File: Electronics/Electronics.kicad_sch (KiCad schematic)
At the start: 54 parts, among them J1 MOT_L, J2 MOT_R, P1 USB_C_Plug_USB2.0, SW1 RST, SW10 BTN8, SW11 BTN9, SW2 BOOT, SW3 BTN1, SW4 BTN2, SW5 BTN3, SW6 BTN4, SW7 BTN5, SW8 BTN6, SW9 BTN7, U1 ESP32-S3-WROOM-1, U2 BMI270, U5 BMI270, U6 NCP1117-3.3_SOT223, U7 NCP1117-3.3_SOT223

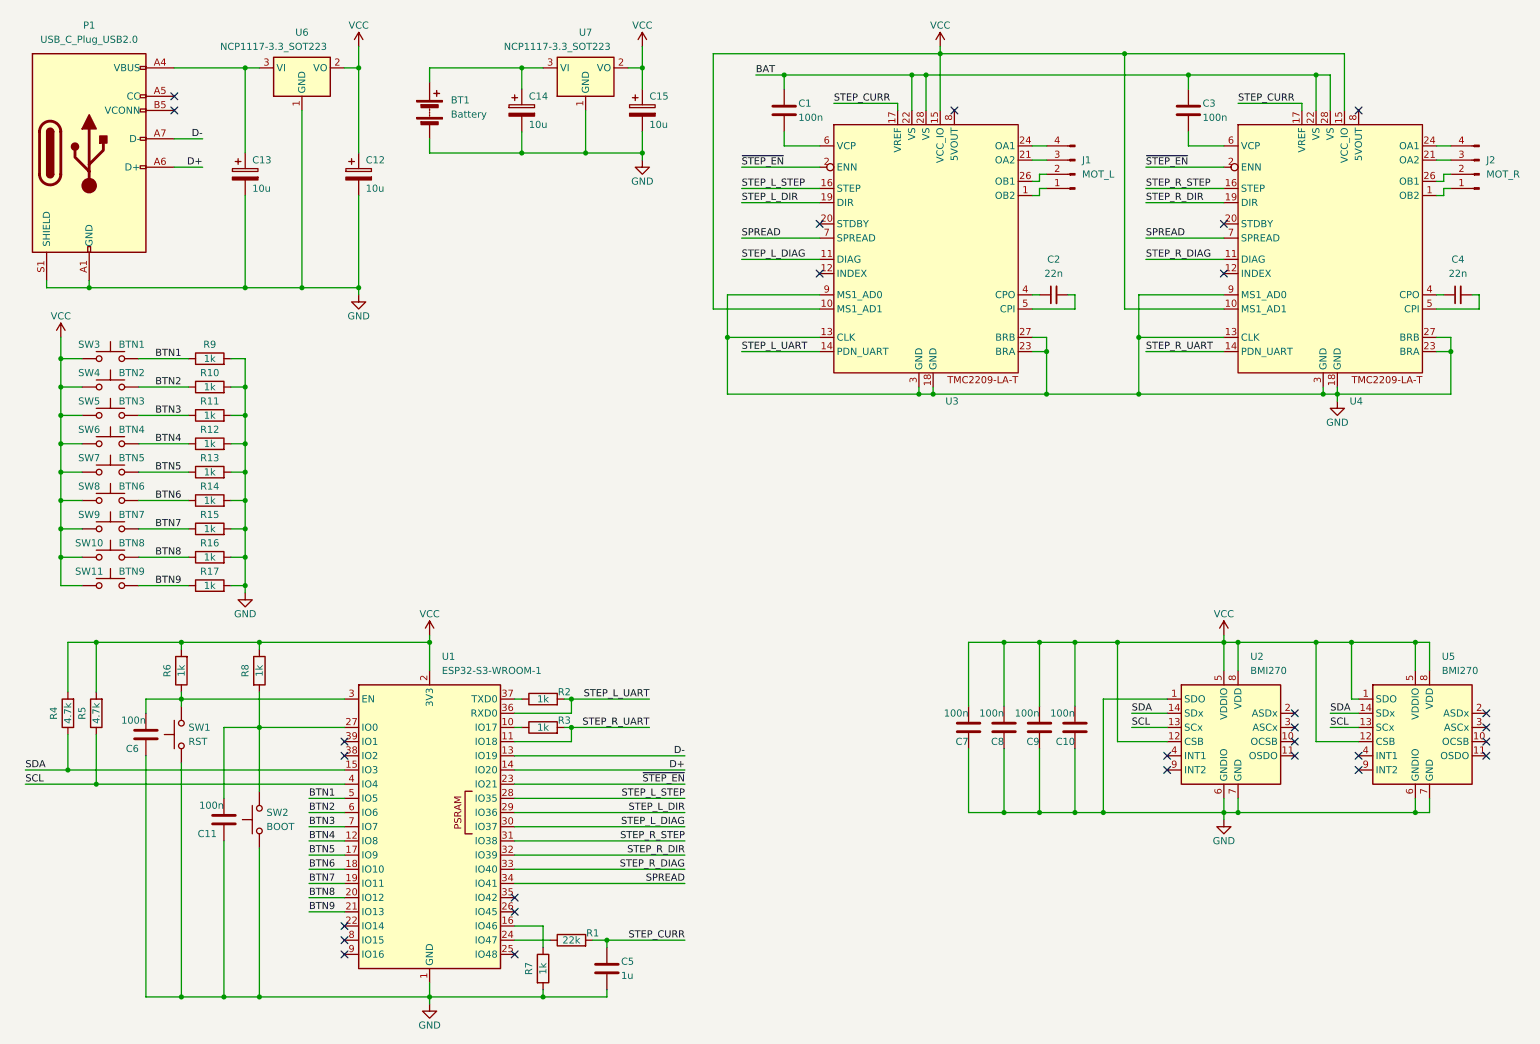
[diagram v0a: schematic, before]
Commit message: oleds
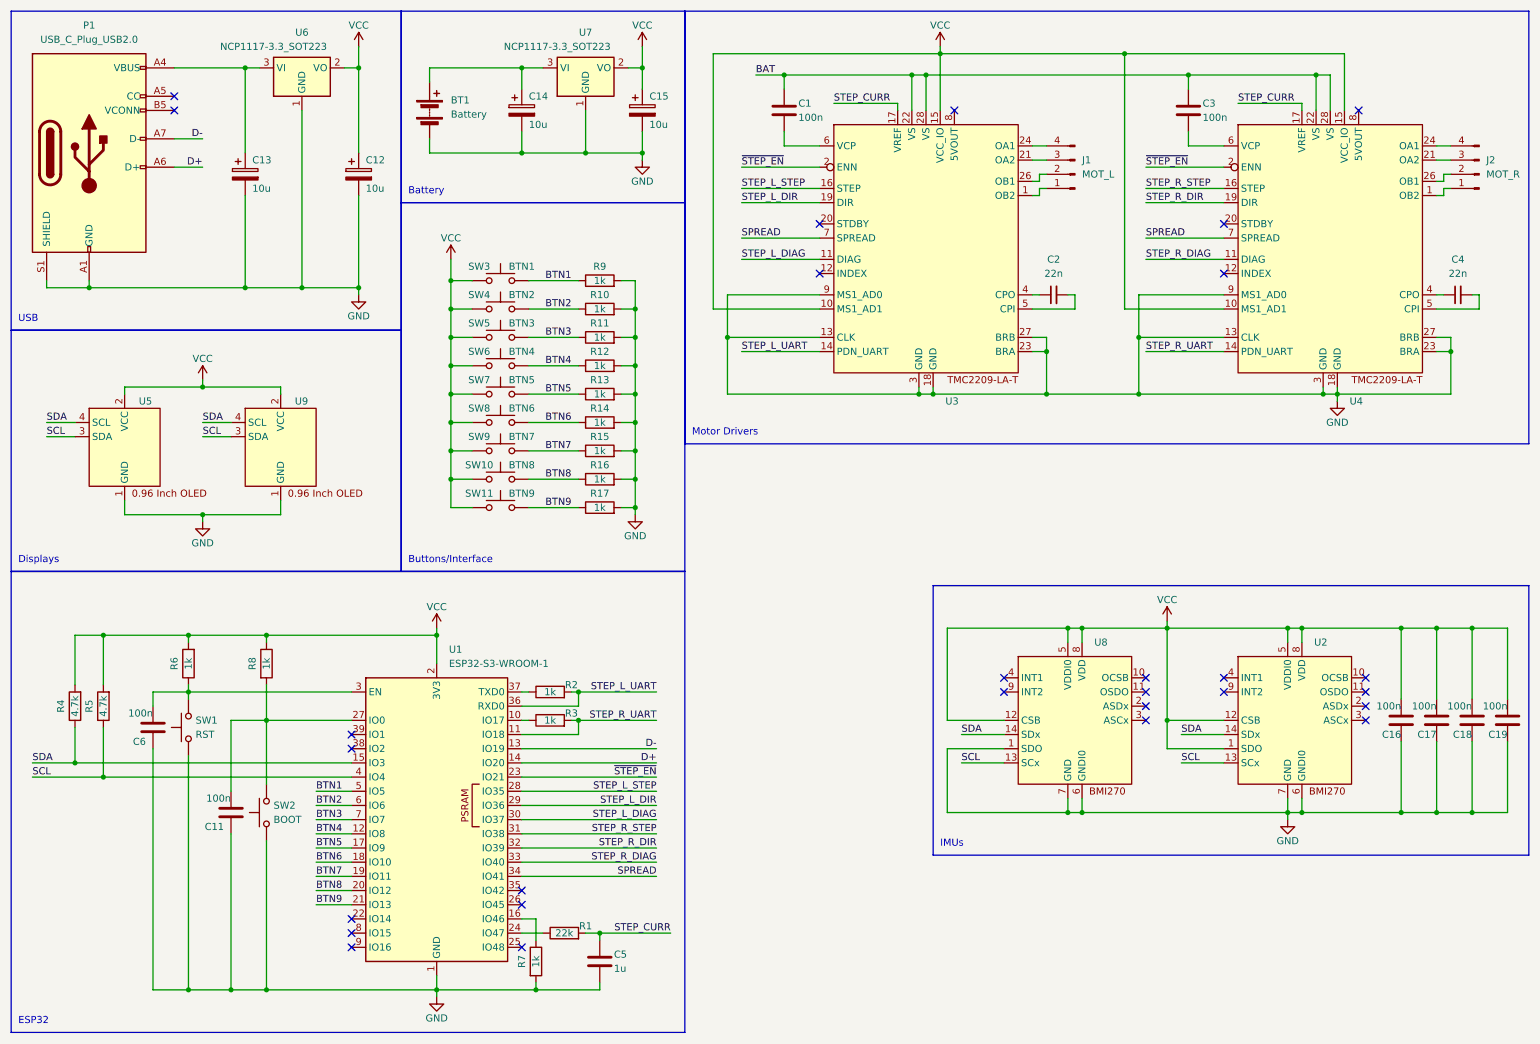
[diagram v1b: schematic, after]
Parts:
- removed C10, C7, C8, C9: 100n, symbol Device:C
- removed U2, U5: BMI270, Package_LGA:Bosch_LGA-14_3x2.5mm_P0.5mm, symbol Sensor_Motion:BMI160
- added C16, C17, C18, C19: 100n, symbol Device:C
- added U2, U8: ~, Package_LGA:Bosch_LGA-14_3x2.5mm_P0.5mm, symbol BMI270:BMI270
- added U5, U9: ~, Connector_PinHeader_2.54mm:PinHeader_1x04_P2.54mm_Vertical, symbol 0.96InchOLED:0.96_Inch_OLED
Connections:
- net GND: now also C16.1, C17.1, C18.1, C19.1, U2.6 (GNDI0), U2.7 (GND), U5.1 (GND), U8.1 (SDO), U8.6 (GNDI0), U8.7 (GND), U9.1 (GND)
- net SCL: now also U2.13 (SCx), U5.3 (SDA), U8.13 (SCx), U9.3 (SDA)
- net SDA: now also U2.14 (SDx), U5.4 (SCL), U8.14 (SDx), U9.4 (SCL)
- net VCC: now also C16.2, C17.2, C18.2, C19.2, U2.1 (SDO), U2.12 (CSB), U2.5 (VDDI0), U2.8 (VDD), U5.2 (VCC), U8.12 (CSB), U8.5 (VDDI0), U8.8 (VDD), U9.2 (VCC)
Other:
- note added: "Battery"
- note added: "Buttons/Interface"
- note added: "Displays"
- note added: "ESP32"
- note added: "IMUs"
- note added: "Motor Drivers"
- note added: "USB"
- moved on the sheet: C11, C5, C6, R1, R10, R11, R12, R13, R14, R15, R16, R17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
